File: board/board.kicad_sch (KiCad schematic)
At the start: 38 parts, among them J1 Conn_01x25_Socket, J2 Conn_01x25_Socket, J5 PJ-320B, J6 Screw_Terminal_01x02, J7 Screw_Terminal_01x02, J8 Screw_Terminal_01x02

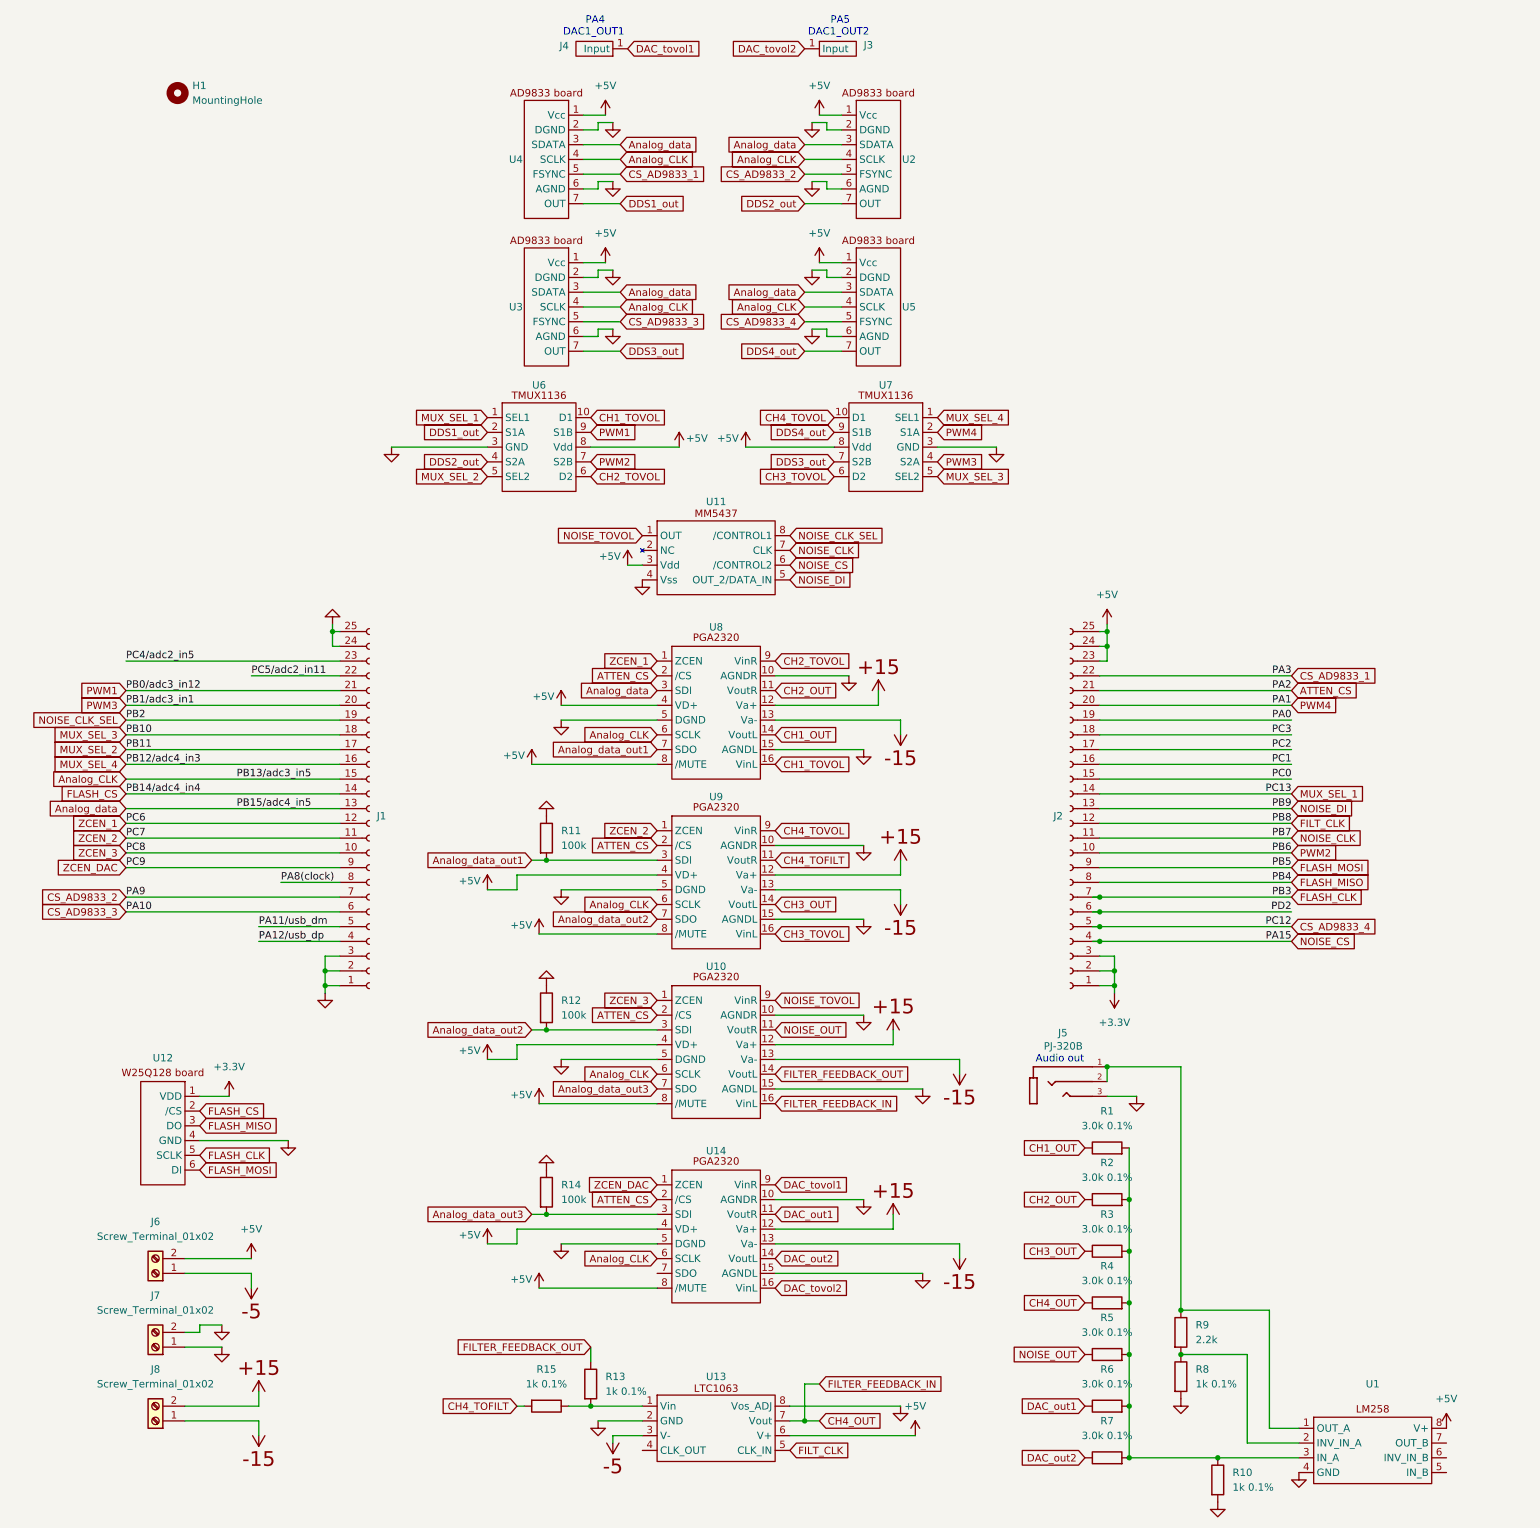
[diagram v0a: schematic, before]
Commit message: add caps on power lines, start tracing
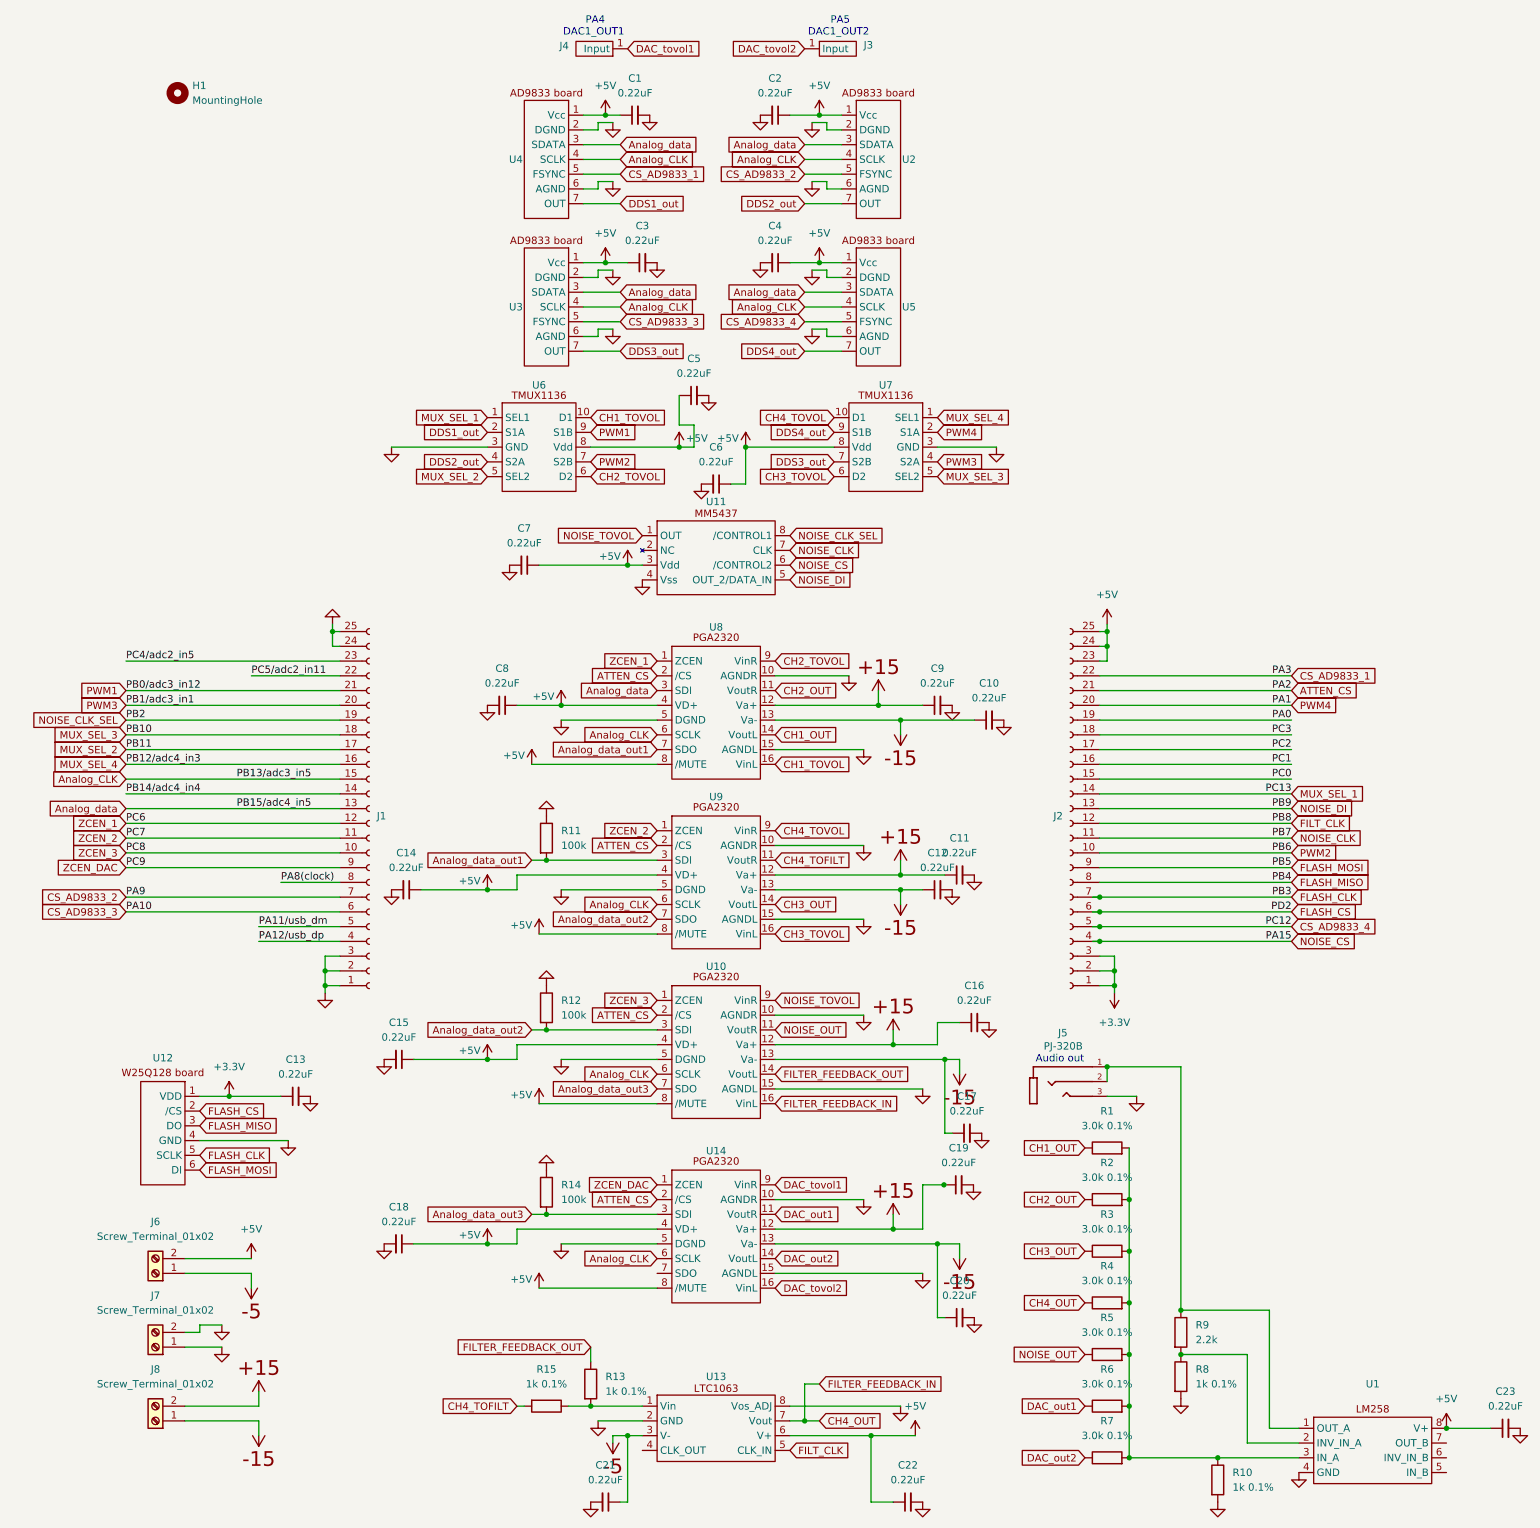
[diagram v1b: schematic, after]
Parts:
- added C1, C10, C11, C12, C13, C14, C15, C16, C17, C18, C19, C2, C20, C21, C22, C23, C3, C4, C5, C6, C7, C8, C9: 0.22uF_0603_25V, 4ms_Capacitor:C_0603, symbol 4ms_Capacitor:0.22uF_0603_25V
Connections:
- net PD2 is gone; now on net FLASH_CS: J2.6 (Pin_6)
- net +3.3V: now also C13.1
- net +5V: now also C1.1, C14.1, C15.1, C18.1, C2.1, C22.1, C23.1, C3.1, C4.1, C5.1, C6.1, C7.1, C8.1
- net FLASH_CS: no longer J1.14 (Pin_14)
- net GND: now also C1.2, C10.2, C11.2, C12.2, C13.2, C14.2, C15.2, C16.2, C17.2, C18.2, C19.2, C2.2, C20.2, C21.2, C22.2, C23.2, C3.2, C4.2, C5.2, C6.2, C7.2, C8.2, C9.2
- net P,+15: now also C11.1, C16.1, C19.1, C9.1
- net P,-15: now also C10.1, C12.1, C17.1, C20.1
- net P,-5: now also C21.1
- new net PB14/adc4_in4: J1.14 (Pin_14)
